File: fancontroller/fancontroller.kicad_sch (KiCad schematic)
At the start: 43 parts, among them J1 Power, J2 Serial Conn, M1 FAN0, M2 FAN0, M3 FAN0, M4 FAN0, M5 FAN0, M6 FAN0, Q1 AO3400A, Q10 AO3401A, Q11 AO3400A, Q12 AO3401A, Q2 AO3401A, Q3 AO3400A, Q4 AO3401A, Q5 AO3400A, Q6 AO3401A, Q7 AO3400A, Q8 AO3401A, Q9 AO3400A, SW1 SW_Push, U2 ESP32-WROOM-32, U3 AMS1117-3.3

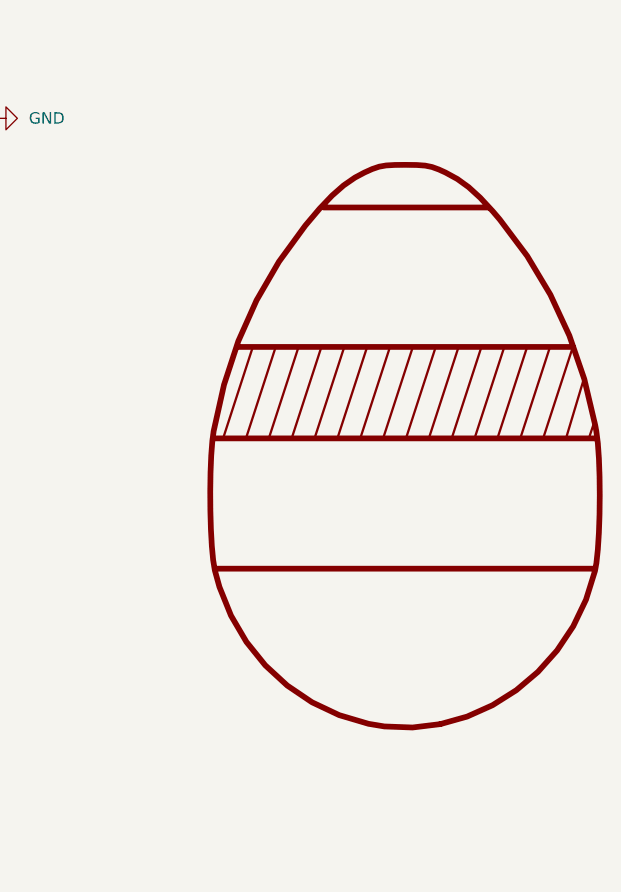
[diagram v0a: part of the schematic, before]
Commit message: prepare to start dev on v1.2
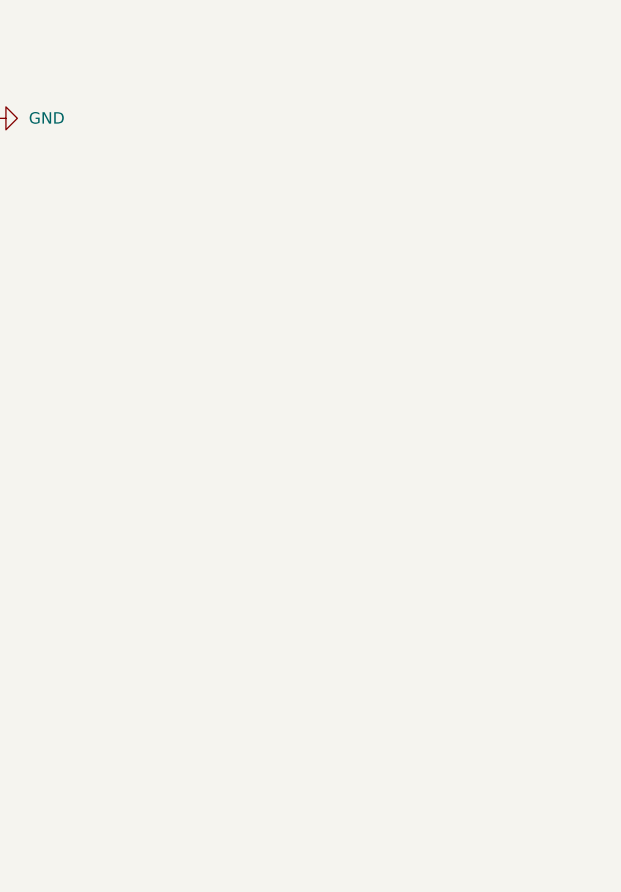
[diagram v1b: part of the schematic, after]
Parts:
- removed SYM1: SYM_EasterEgg_42x60mm, Symbol:Symbol_GNU-Logo_SilkscreenTop, symbol Graphic:SYM_EasterEgg_42x60mm
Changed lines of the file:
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@@
-	)
-	(symbol
-		(lib_id "Graphic:SYM_EasterEgg_42x60mm")
-		(at 240.03 144.78 0)
-		(unit 1)
-		(exclude_from_sim yes)
-		(in_bom no)
-		(on_board yes)
-		(dnp no)
-		(fields_autoplaced yes)
-		(property "Reference" "SYM1"
-			(at 240.03 144.78 0)
-			(effects
-				(font
-					(size 1.27 1.27)
-				)
-				(hide yes)
-			)
-		)
-		(property "Value" "SYM_EasterEgg_42x60mm"
-			(at 240.03 144.78 0)
-			(effects
-				(font
-					(size 1.27 1.27)
-				)
-				(hide yes)
-			)
-		)
-		(property "Footprint" "Symbol:Symbol_GNU-Logo_SilkscreenTop"
-			(at 240.03 148.59 0)
-			(effects
-				(font
-					(size 1.27 1.27)
-				)
-				(hide yes)
-			)
-		)
-		(property "Datasheet" "https://eur-lex.europa.eu/LexUriServ/LexUriServ.do?uri=OJ:L:2013:347:0671:0854:de:PDF"
-			(at 240.03 151.13 0)
-			(effects
-				(font
-					(size 1.27 1.27)
-				)
-				(hide yes)
-			)
-		)
-		(property "Description" "EasterEgg, ClassA, Medium Size"
-			(at 240.03 144.78 0)
-			(effects
-				(font
-					(size 1.27 1.27)
-				)
-				(hide yes)
-			)
-		)
-		(property "LCSC Part #" ""
-			(at 240.03 144.78 0)
-			(effects
-				(font
-					(size 1.27 1.27)
-				)
-				(hide yes)
-			)
-		)
-		(property "JLCPCB Rotation Offset" ""
-			(at 240.03 144.78 0)
-			(effects
-				(font
-					(size 1.27 1.27)
-				)
-				(hide yes)
-			)
-		)
-		(instances
-			(project ""
-				(path "/0224fd83-71fd-467a-bea0-55e2843206f4"
-					(reference "SYM1")
-					(unit 1)
-				)
-			)
-		)
 	)
 	(symbol
